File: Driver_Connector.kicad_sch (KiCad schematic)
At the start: 3 parts, among them J11 Input, J5 Driver, J6 Measurements

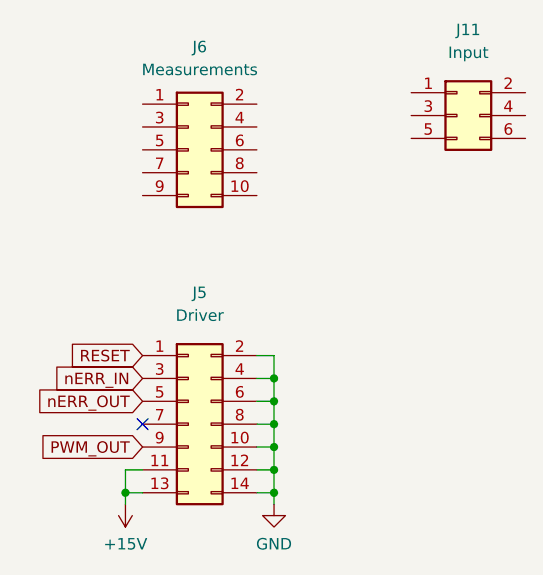
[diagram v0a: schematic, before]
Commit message: Первая версия в производство
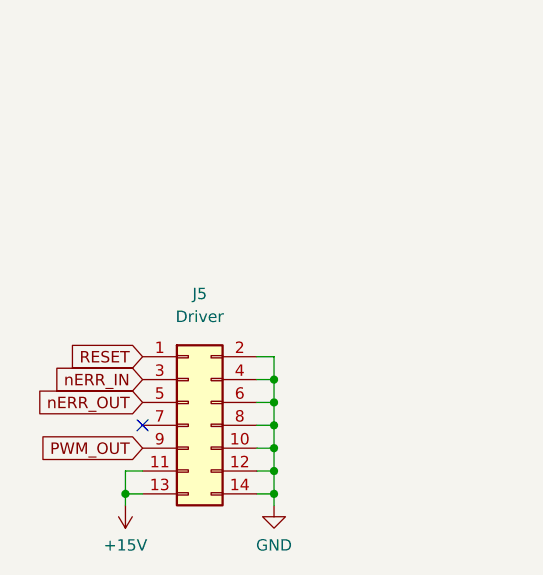
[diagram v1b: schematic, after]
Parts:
- removed J11: Input, Connector_Molex:Molex_Micro-Fit_3.0_43045-0600_2x03_P3.00mm_Horizontal, symbol Connector_Generic:Conn_02x03_Odd_Even
- removed J6: Measurements, Connector_IDC:IDC-Header_2x05_P2.54mm_Vertical, symbol Connector_Generic:Conn_02x05_Odd_Even
